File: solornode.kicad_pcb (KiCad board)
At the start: 2 copper layers, 77 parts, among them J1 Conn_01x06, Q1 Q_NMOS_GDS, Q4 Q_PNP_BCE, Q5 Q_NPN_BCE, SW1 SW_Push, U1 LM358, U2 OC5864, U3 PY32F003F1xUx, U4 MAX485E, U5 SGM2033-5.0

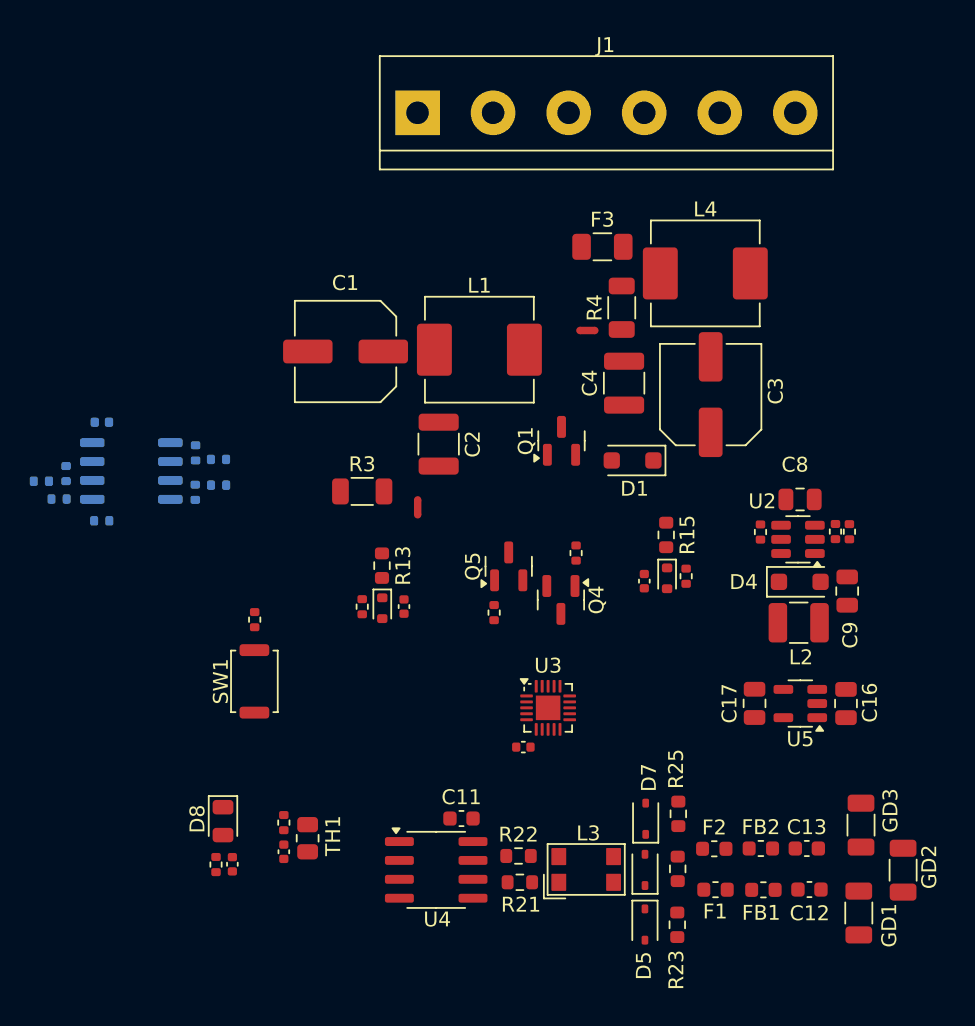
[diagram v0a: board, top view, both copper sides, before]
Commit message: PCB布局，划定边框
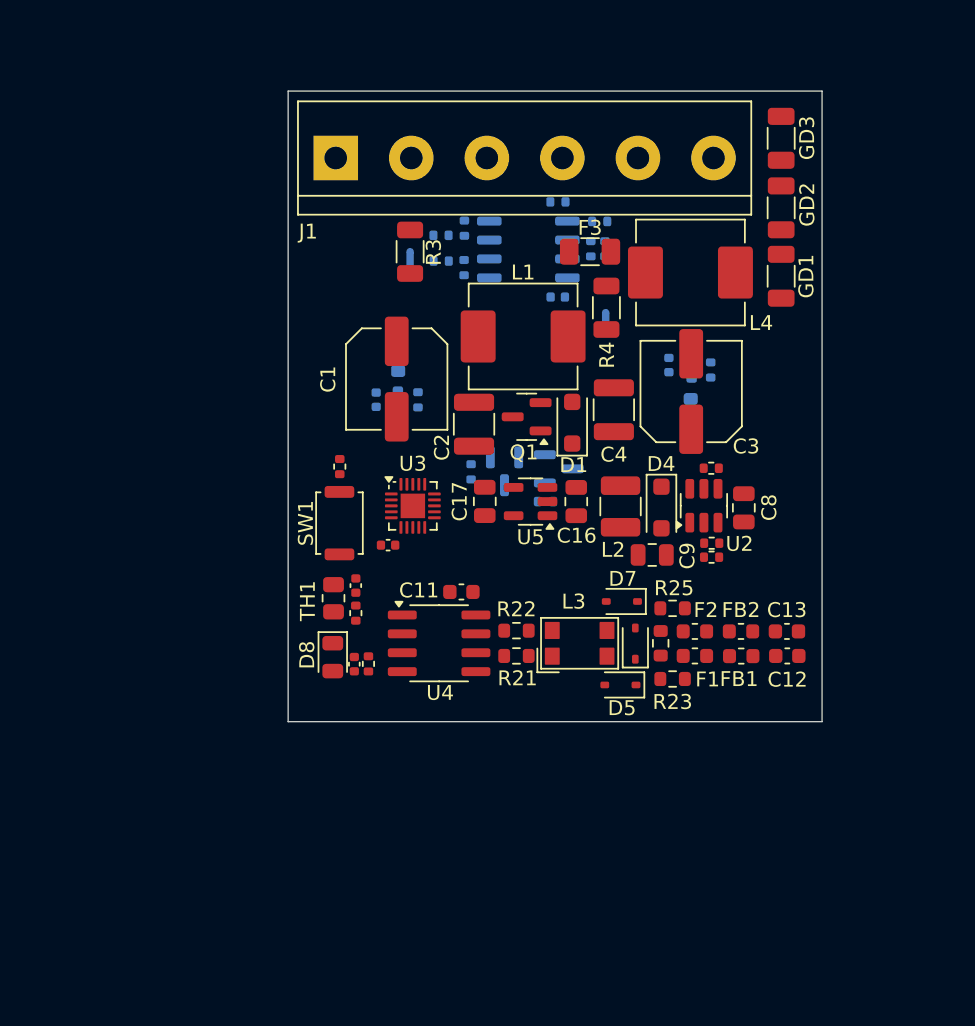
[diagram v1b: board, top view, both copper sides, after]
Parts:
- C6, C7, D2, D3, NT1, NT2, Q4, Q5, R1, R13, R14, R15, R16, R2: moved to B.Cu
- moved GD3 46.5 mm to (145.8, 60.1)
- moved GD2 45.3 mm to (145.8, 64.8)
- moved GD1 43.1 mm to (145.8, 69.3)
- moved R10 41.0 mm to (133.9, 67.5), turned to 90 degrees
- moved R9 40.9 mm to (133.6, 65.7), turned to 180 degrees
- moved R12 38.4 mm to (132.9, 67.5), turned to -90 degrees
- moved R11 37.4 mm to (130.7, 64.3), turned to 180 degrees
- moved C5 31.8 mm to (130.7, 70.8), turned to 180 degrees
- moved U1 30.6 mm to (128.8, 67.5), turned to 0 degrees
- moved R8 25.4 mm to (124.5, 66.1), turned to 90 degrees
- moved C16 22.7 mm to (132.0, 84.5)
- moved C17 22.7 mm to (125.8, 84.5)
- moved U5 22.7 mm to (128.9, 84.5)
- moved R7 22.5 mm to (122.9, 66.6), turned to 0 degrees
- moved R6 21.9 mm to (124.4, 68.8), turned to -90 degrees
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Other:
- board outline added: 35.9 x 42.4 mm
